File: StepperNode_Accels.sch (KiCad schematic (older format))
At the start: 20 parts

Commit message: First Revision -
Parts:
- removed C? (x12): 100nF, symbol C
- removed R? (x4): 10K, symbol R
- added C12, C13, C14, C15, C16, C17, C18, C19, C20, C21, C22, C23: C_100nF_50V, RLOOP_FOOTPRINTS:rLoop_C_0603, symbol C_100nF_50V
- added R1, R2, R3, R4: 10K, RLOOP_FOOTPRINTS:rLoop_R_0603, symbol 10K
- gave numbers to parts that had none: 4
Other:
- moved on the sheet: U6, U7, U8, U9

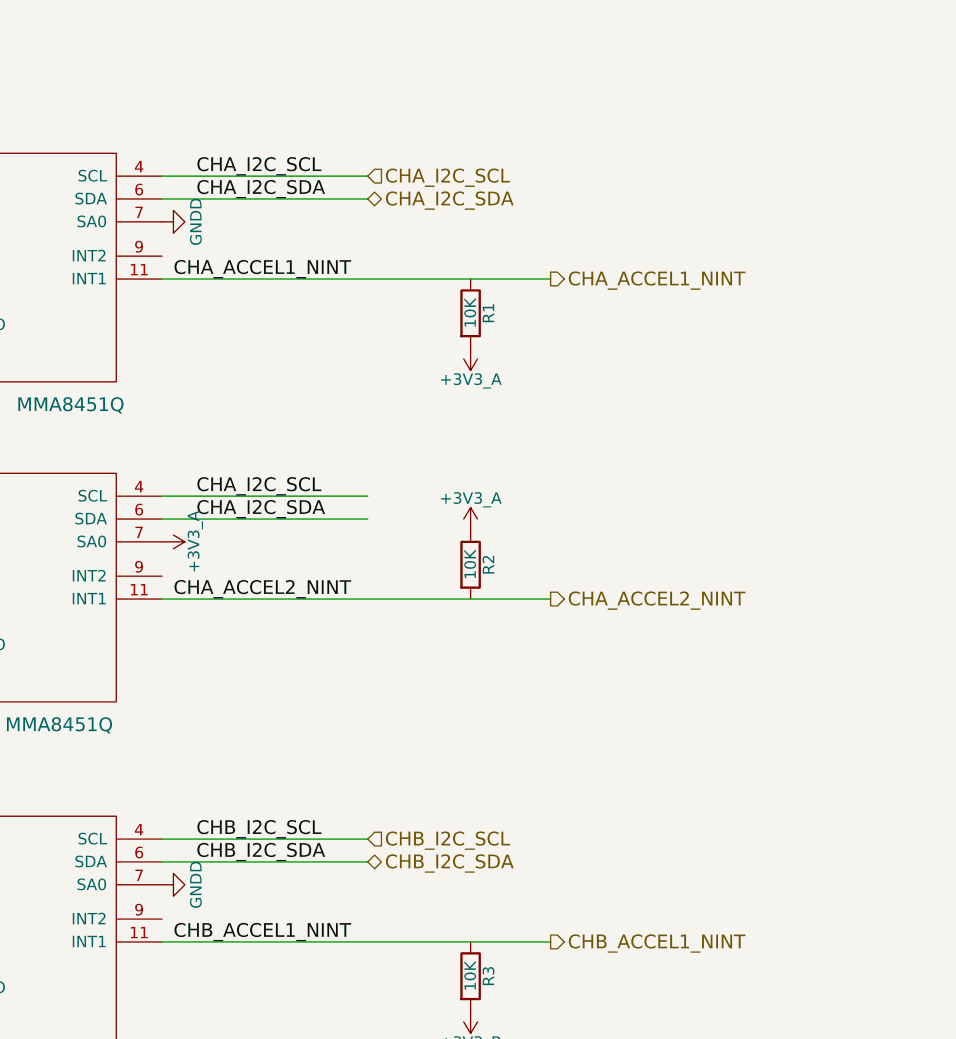
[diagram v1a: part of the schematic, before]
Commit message: Update per design review.
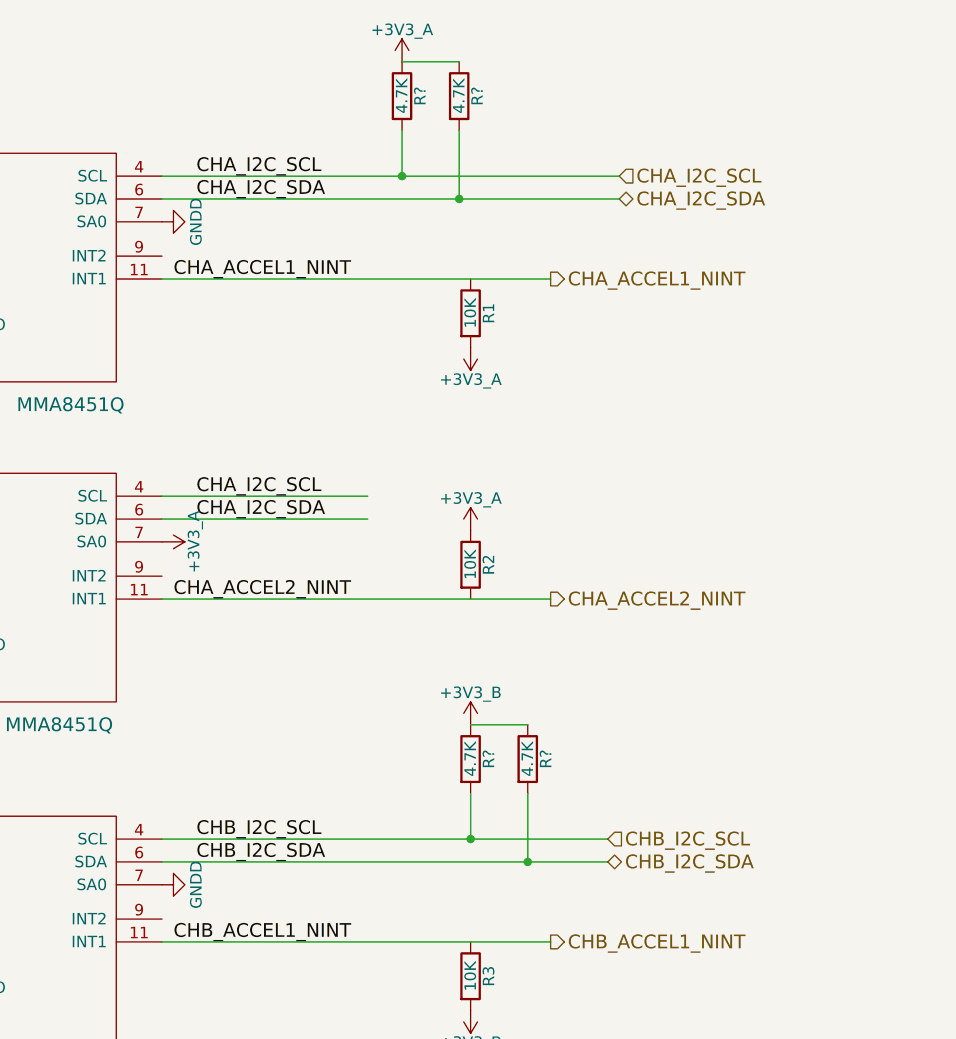
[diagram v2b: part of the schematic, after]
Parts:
- added R? (x4): 4.7K, RLOOP_FOOTPRINTS:rLoop_R_0603, symbol 4.7K
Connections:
- wire segments 20 -> 26
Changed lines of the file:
@@
 Title "Accelerometers"
 Date ""
-Rev "1"
+Rev "2"
 Comp ""
 Comment1 ""
@@
 $EndComp
 Wire Wire Line
-	5900 1700 6800 1700
-Wire Wire Line
-	5900 1800 6800 1800
+	5900 1700 7900 1700
+Wire Wire Line
+	5900 1800 7900 1800
 Text Label 6050 1700 0    60   ~ 0
 CHA_I2C_SCL
@@
 $EndComp
 Wire Wire Line
-	5900 4600 6800 4600
-Wire Wire Line
-	5900 4700 6800 4700
+	5900 4600 7850 4600
+Wire Wire Line
+	5900 4700 7850 4700
 Text Label 6050 4600 0    60   ~ 0
 CHB_I2C_SCL
@@
 Text Label 5950 6450 0    60   ~ 0
 CHB_ACCEL2_NINT
-Text HLabel 6800 1700 2    60   Input ~ 0
+Text HLabel 7900 1700 2    60   Input ~ 0
 CHA_I2C_SCL
-Text HLabel 6800 1800 2    60   BiDi ~ 0
+Text HLabel 7900 1800 2    60   BiDi ~ 0
 CHA_I2C_SDA
 Text HLabel 7600 2150 2    60   Output ~ 0
@@
 	0    -1   -1   0
 $EndComp
-Text HLabel 6800 4600 2    60   Input ~ 0
+Text HLabel 7850 4600 2    60   Input ~ 0
 CHB_I2C_SCL
-Text HLabel 6800 4700 2    60   BiDi ~ 0
+Text HLabel 7850 4700 2    60   BiDi ~ 0
 CHB_I2C_SDA
 $Comp
@@
 	1    0    0    -1
 $EndComp
+$Comp
+L 4.7K R?
+U 1 1 575CC544
+P 6950 1350
+F 0 "R?" V 7030 1350 50  0000 C CNN
+F 1 "4.7K" V 6950 1350 50  0000 C CNN
+F 2 "RLOOP_FOOTPRINTS:rLoop_R_0603" V 6880 1350 50  0001 C CNN
+F 3 "" H 6950 1350 50  0000 C CNN
+	1    6950 1350
+	1    0    0    -1
+$EndComp
+$Comp
+L 4.7K R?
+U 1 1 575CC5B1
+P 7200 1350
+F 0 "R?" V 7280 1350 50  0000 C CNN
+F 1 "4.7K" V 7200 1350 50  0000 C CNN
+F 2 "RLOOP_FOOTPRINTS:rLoop_R_0603" V 7130 1350 50  0001 C CNN
+F 3 "" H 7200 1350 50  0000 C CNN
+	1    7200 1350
+	1    0    0    -1
+$EndComp
+$Comp
+L +3V3_A #PWR?
+U 1 1 575CC5CD
+P 6950 1200
+F 0 "#PWR?" H 6950 1050 50  0001 C CNN
+F 1 "+3V3_A" H 6950 1340 50  0000 C CNN
+F 2 "" H 6950 1200 60  0000 C CNN
+F 3 "" H 6950 1200 60  0000 C CNN
+	1    6950 1200
+	1    0    0    -1
+$EndComp
+Wire Wire Line
+	6950 1200 7200 1200
+Wire Wire Line
+	6950 1500 6950 1700
+Connection ~ 6950 1700
+Wire Wire Line
+	7200 1500 7200 1800
+Connection ~ 7200 1800
+$Comp
+L 4.7K R?
+U 1 1 575CC8DB
+P 7250 4250
+F 0 "R?" V 7330 4250 50  0000 C CNN
+F 1 "4.7K" V 7250 4250 50  0000 C CNN
+F 2 "RLOOP_FOOTPRINTS:rLoop_R_0603" V 7180 4250 50  0001 C CNN
+F 3 "" H 7250 4250 50  0000 C CNN
+	1    7250 4250
+	1    0    0    -1
+$EndComp
+$Comp
+L 4.7K R?
+U 1 1 575CC8E1
+P 7500 4250
+F 0 "R?" V 7580 4250 50  0000 C CNN
+F 1 "4.7K" V 7500 4250 50  0000 C CNN
+F 2 "RLOOP_FOOTPRINTS:rLoop_R_0603" V 7430 4250 50  0001 C CNN
+F 3 "" H 7500 4250 50  0000 C CNN
+	1    7500 4250
+	1    0    0    -1
+$EndComp
+Wire Wire Line
+	7250 4100 7500 4100
+Wire Wire Line
+	7250 4400 7250 4600
+Connection ~ 7250 4600
+Wire Wire Line
+	7500 4400 7500 4700
+Connection ~ 7500 4700
+$Comp
+L +3V3_B #PWR?
+U 1 1 575CCA5D
+P 7250 4100
+F 0 "#PWR?" H 7250 3950 50  0001 C CNN
+F 1 "+3V3_B" H 7250 4240 50  0000 C CNN
+F 2 "" H 7250 4100 60  0000 C CNN
+F 3 "" H 7250 4100 60  0000 C CNN
+	1    7250 4100
+	1    0    0    -1
+$EndComp
